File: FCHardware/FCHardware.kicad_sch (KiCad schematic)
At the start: 43 parts, among them J1 JST-8pin, J3 USB_C_Receptacle_USB2.0_16P, SW3 SW_Push, SW4 SW_Push, U2 MPU-6050, U4 TPSM63603, U5 ESC_Xrotor_65A_4in1, U8 ESP32-S3-MINI-1U, U9 USBLC6-2SC6

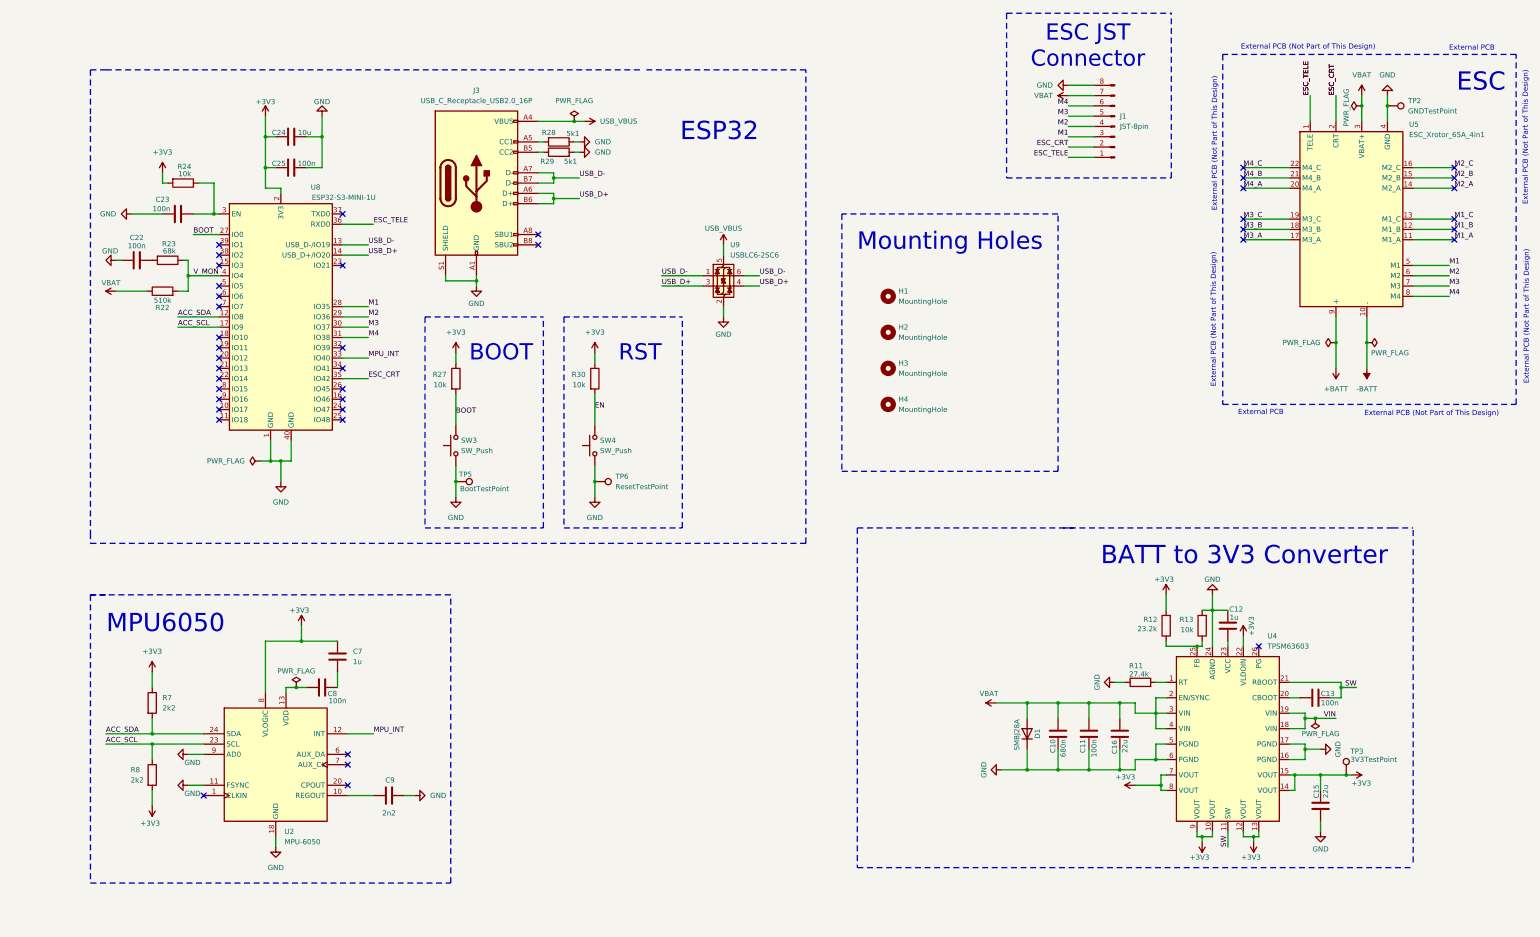
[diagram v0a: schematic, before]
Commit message: Switched to STM mcu and ICM-42688 imu
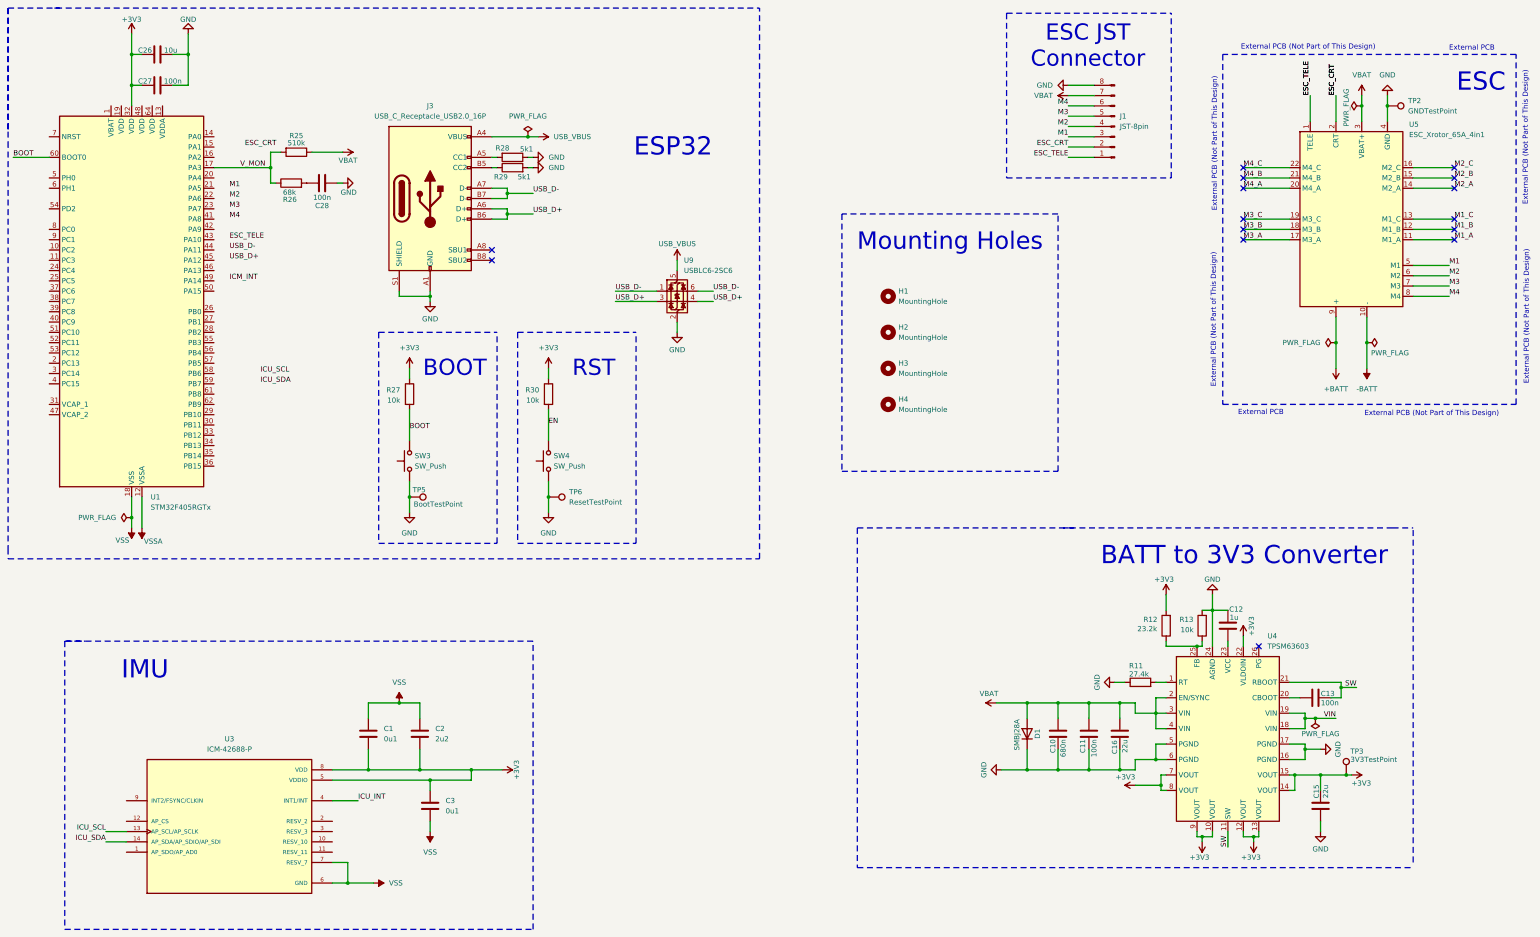
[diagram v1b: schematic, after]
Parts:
- removed C22, C23, C25, C8: 100n, Capacitor_SMD:C_0603_1608Metric_Pad1.08x0.95mm_HandSolder, symbol Device:C
- removed C24: 10u, Capacitor_SMD:C_0805_2012Metric_Pad1.18x1.45mm_HandSolder, symbol Device:C
- removed C7: 1u, Capacitor_SMD:C_0603_1608Metric_Pad1.08x0.95mm_HandSolder, symbol Device:C
- removed C9: 2n2, Capacitor_SMD:C_0603_1608Metric_Pad1.08x0.95mm_HandSolder, symbol Device:C
- removed R22: 510k, Resistor_SMD:R_0603_1608Metric_Pad0.98x0.95mm_HandSolder, symbol Device:R
- removed R23: 68k, Resistor_SMD:R_0603_1608Metric_Pad0.98x0.95mm_HandSolder, symbol Device:R
- removed R24: 10k, Resistor_SMD:R_0603_1608Metric_Pad0.98x0.95mm_HandSolder, symbol Device:R
- removed R7, R8: 2k2, Resistor_SMD:R_0603_1608Metric_Pad0.98x0.95mm_HandSolder, symbol Device:R
- removed U2: MPU-6050, Sensor_Motion:InvenSense_QFN-24_4x4mm_P0.5mm, symbol Sensor_Motion:MPU-6050
- removed U8: ESP32-S3-MINI-1U, RF_Module:ESP32-S3-WROOM-1U, symbol Custom_ESP32_Library:ESP32-S3-MINI-1U
- added C1, C3: 0u1, symbol Device:C
- added C2: 2u2, symbol Device:C
- added C26: 10u, Capacitor_SMD:C_0805_2012Metric_Pad1.18x1.45mm_HandSolder, symbol Device:C
- added C27, C28: 100n, Capacitor_SMD:C_0603_1608Metric_Pad1.08x0.95mm_HandSolder, symbol Device:C
- added R25: 510k, Resistor_SMD:R_0603_1608Metric_Pad0.98x0.95mm_HandSolder, symbol Device:R
- added R26: 68k, Resistor_SMD:R_0603_1608Metric_Pad0.98x0.95mm_HandSolder, symbol Device:R
- added U1: STM32F405RGTx, Package_QFP:LQFP-64_10x10mm_P0.5mm, symbol MCU_ST_STM32F4:STM32F405RGTx
- added U3: ICM-42688-P, ICM-42688-P:PQFN50P300X250X97-14N, symbol ICM-42688-P:ICM-42688-P
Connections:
- net +3V3: now also C1.2, C2.2, C26.2, C27.2, C3.1, U1.32 (VDD), U3.5 (VDDIO), U3.8 (VDD)
- net BOOT: now also U1.60 (BOOT0)
- net GND: now also C26.1, C27.1, C28.1
- net VBAT: now also R25.1
- net V_MON: now also R25.2, R26.1, U1.17 (PA3)
- new net: C28.2, R26.2
- new net ICU_INT: U3.4 (INT1/INT)
- new net ICU_SCL: U3.13 (AP_SCL/AP_SCLK)
- new net ICU_SDA: U3.14 (AP_SDA/AP_SDIO/AP_SDI)
- new net VSS: C1.1, C2.1, C3.2, U1.18 (VSS), U1.63 (VSS), U3.6 (GND), U3.7 (RESV_7)
- new net VSSA: U1.12 (VSSA)
- no-connect marks 42 -> 15
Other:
- note added: "IMU"
- note removed: "MPU6050"
- moved on the sheet: J3, R27, R28, R29, R30, SW3, SW4, TP5, TP6, U9
